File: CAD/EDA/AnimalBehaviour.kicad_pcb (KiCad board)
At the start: 2 copper layers, 105 x 76.5 mm, 26 parts, among them J1 SSR_INPUT, J10 JSolenoid, J11 LED, J12 Cam, J13 Imaging, J14 Ext Supp, J2 SSR OUT, J3 StimCurrentInject, J4 StimIsoIN, J5 StimIsoIN, J6 Imaging, J7 CAM, J8 TONE, J9 TONE, Q1 IRF540N, U1 4N35

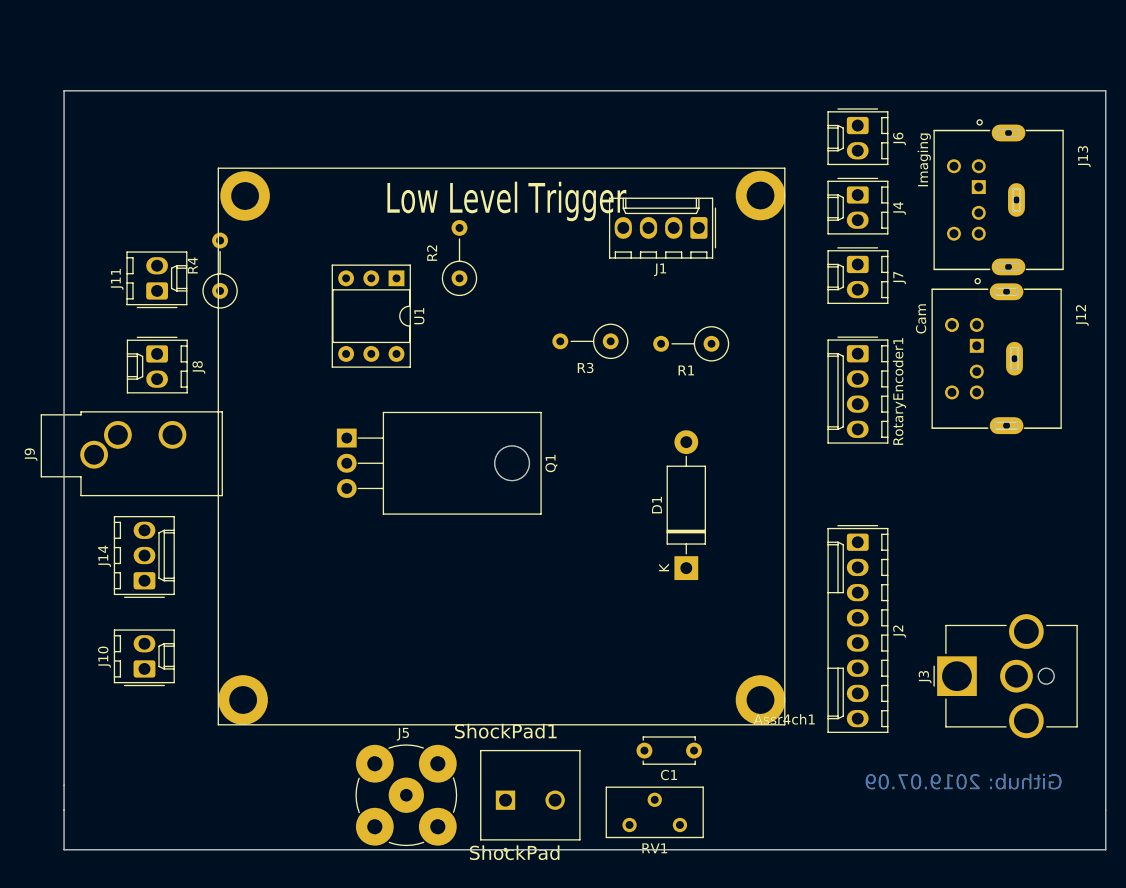
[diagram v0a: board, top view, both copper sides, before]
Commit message: version 2019.07.09
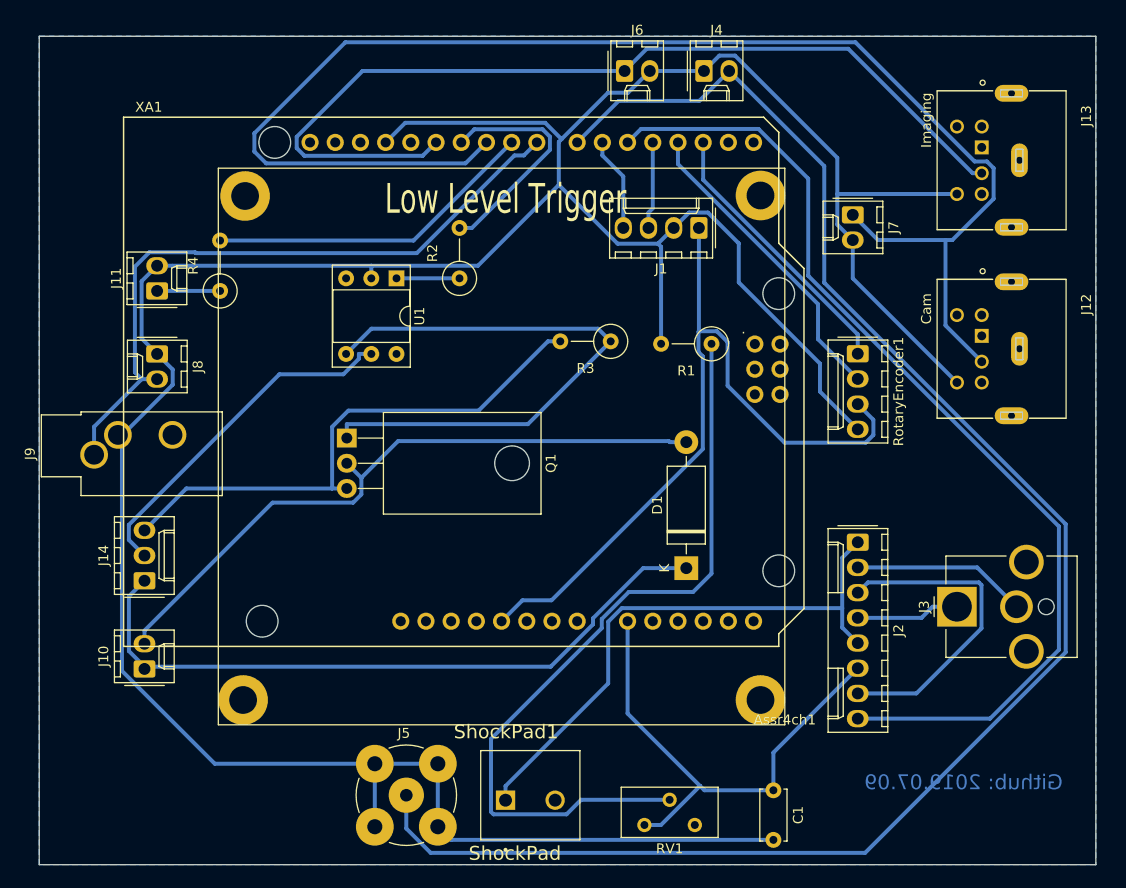
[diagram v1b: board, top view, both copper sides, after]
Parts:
- added XA1: Arduino_Uno_Shield, Arduino:Arduino_Uno_Shield, F.Cu at (116.0, 126.0)
- moved J6 24.1 mm to (166.5, 68.0), turned to 0 degrees
- moved J4 19.9 mm to (174.5, 68.0), turned to 0 degrees
- moved C1 8.94 mm to (181.5, 140.5), turned to 270 degrees
- moved J3 7.00 mm to (200.0, 122.0)
- moved J7 5.02 mm to (189.5, 82.5)
- moved J13 4.01 mm to (204.5, 77.0)
- moved RV1 1.50 mm to (168.5, 144.0)
- moved J12 1.12 mm to (204.5, 96.0)
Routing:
- net DGND: track 0.00 -> 329.6 mm
- net ShockStimIsolator: track 0.00 -> 170.1 mm
- net CamTTL: track 0.00 -> 144.0 mm
- net ShockPWM: track 0.00 -> 102.0 mm
- net ImagingTrig: track 0.00 -> 94.0 mm
- net Net-(R1-Pad1): track 0.00 -> 78.9 mm
- net 5V: track 0.00 -> 78.9 mm
- net EX_12V: track 0.00 -> 69.3 mm
- net TONE+: track 0.00 -> 68.6 mm
- net Net-(D1-Pad2): track 0.00 -> 66.9 mm
- net Net-(Q1-Pad1): track 0.00 -> 59.7 mm
- net PAD-: track 0.00 -> 57.9 mm
- net AGND: track 0.00 -> 54.9 mm
- net ShockRead: track 0.00 -> 50.3 mm
- net EX_5V: track 0.00 -> 35.6 mm
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- added copper zone on B.Cu, net DGND
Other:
- board size 105 x 76.5 mm -> 106.5 x 83.5 mm
